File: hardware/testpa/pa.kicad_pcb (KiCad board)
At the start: 4 copper layers, 50 x 50 mm, 63 parts, among them CN1 CONN_01X02, J1 JNC, J2 JNC, Q1 LDMOS, Q2 LDMOS, T1 TRANSF4CTS, T2 1:1 Z, U1 LP2985

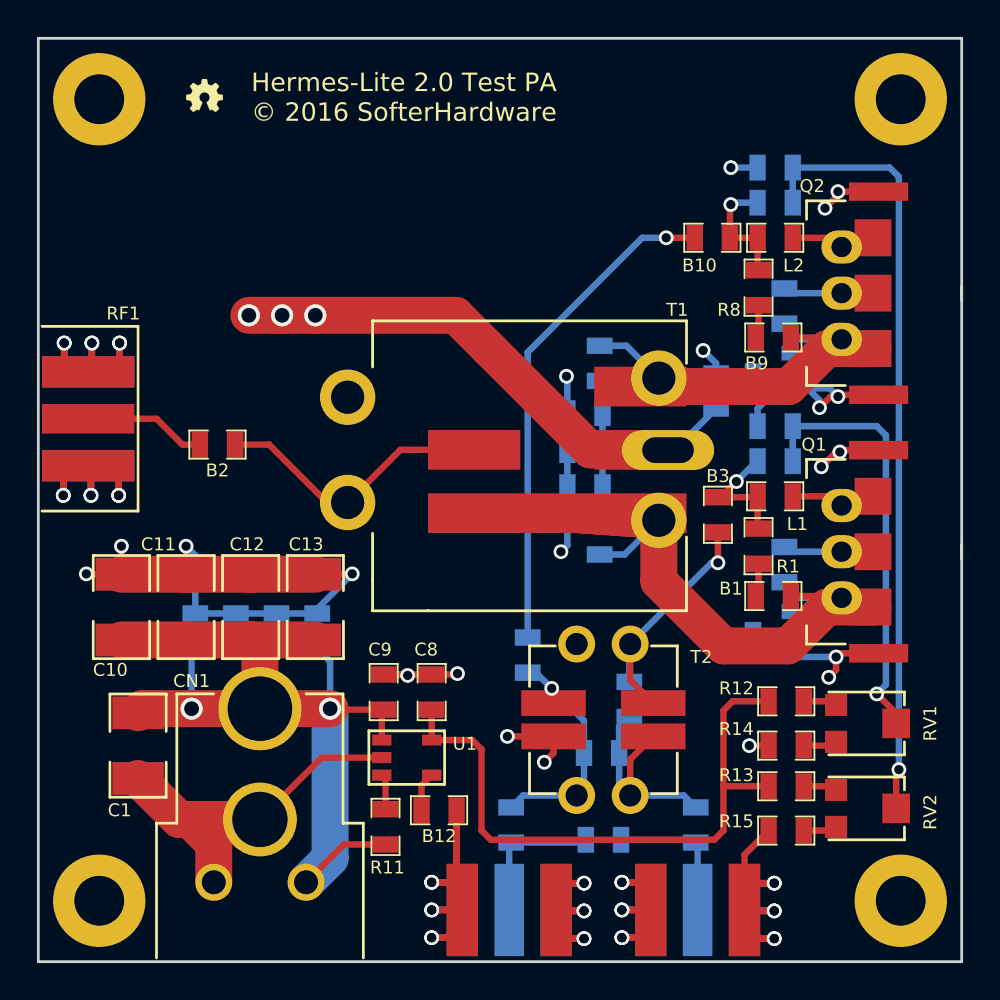
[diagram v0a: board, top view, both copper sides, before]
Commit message: Final PCBs, added gerber
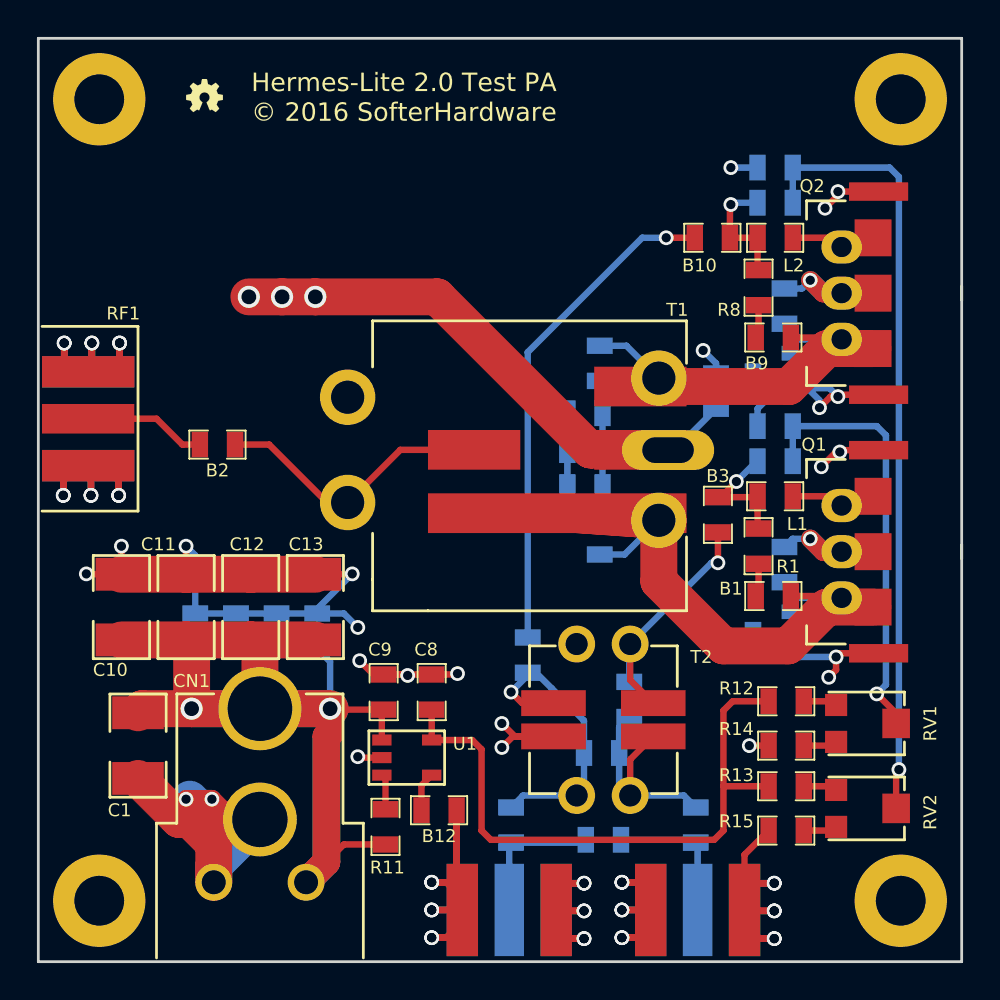
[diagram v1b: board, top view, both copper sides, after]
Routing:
- net /Vpa: track 147.2 -> 159.2 mm
- net GND: track 290.5 -> 302.3 mm, vias 57 -> 62
- net Net-(J2-Pad2): track 13.0 -> 16.1 mm
- added copper zone on B.Cu, net GND
- added copper zone on F.Cu, net GND
